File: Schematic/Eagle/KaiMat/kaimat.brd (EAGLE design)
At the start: 60.1 x 110.5 mm, 35 parts, among them IC1 MCP6004-E_P

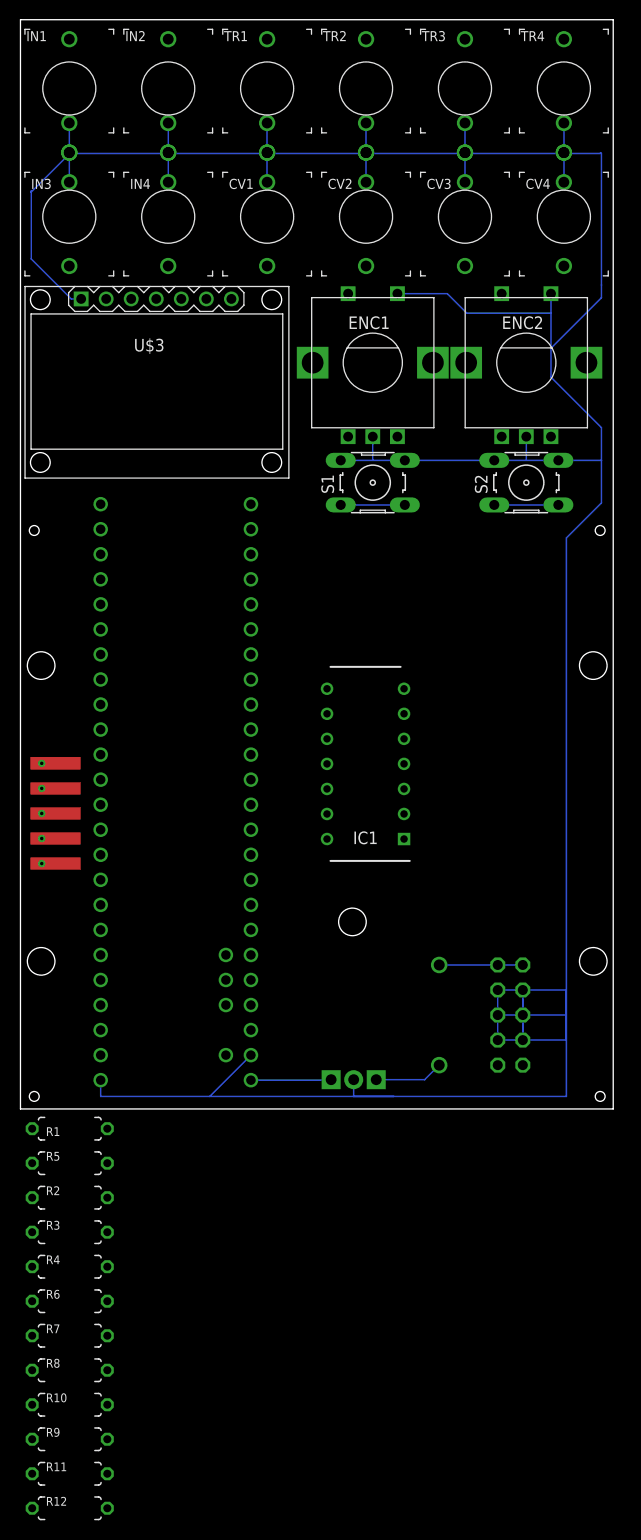
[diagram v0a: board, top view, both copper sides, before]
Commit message: improved schematic
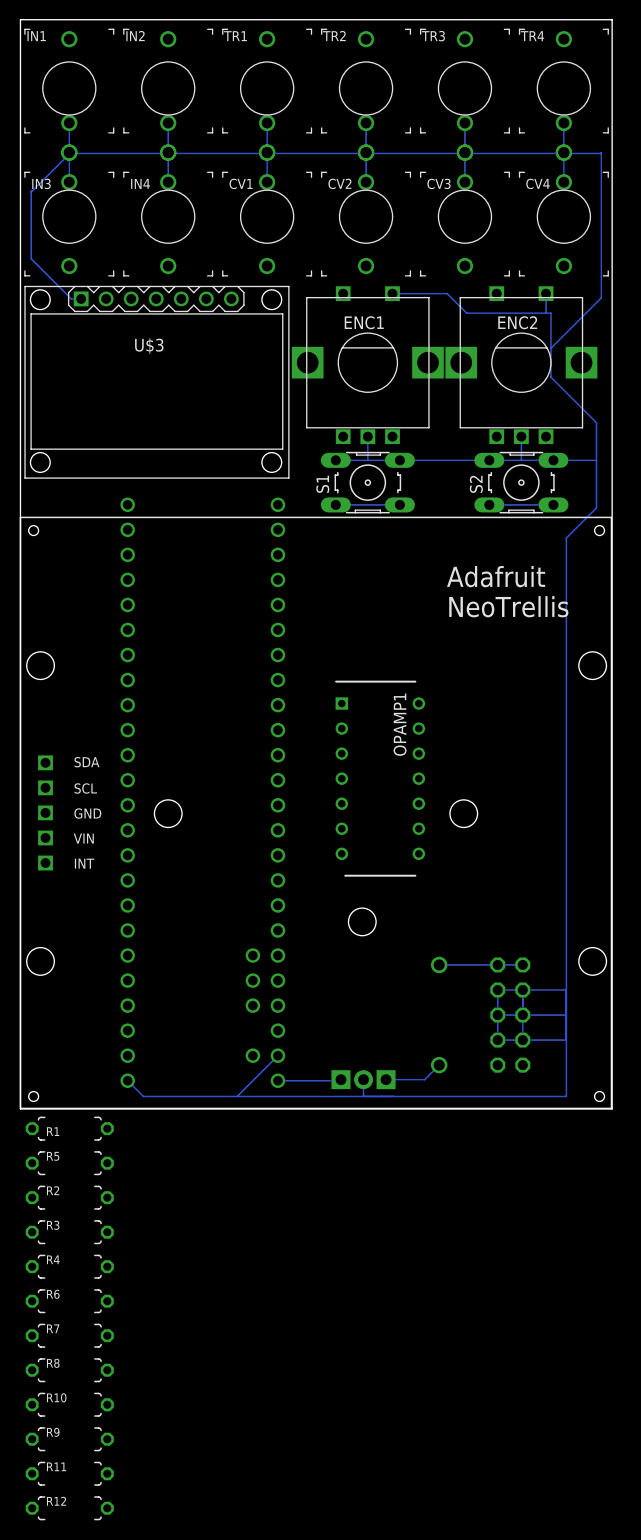
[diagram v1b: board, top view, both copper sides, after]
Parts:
- removed IC1: MCP6004-E_P, mcp6004-e_p:DIP781W56P254L1918H533Q14N
- removed JP1: (no value), microbuilder:5P_EDGECONNECT
- added OPAMP1: MCP6004-E_P, mcp6004-e_p:DIP781W56P254L1918H533Q14N
- added U$4: NEOTRELLISKAIMAT2, Adafruit Trellis:NEOTRELLISKAIMAT2
- moved U$1 2.74 mm to (18.5, 30.8)
- moved U$2 1.00 mm to (34.9, 12.6)
- moved ENC1 0.50 mm to (35.2, 75.7)
- moved ENC2 0.50 mm to (50.8, 75.7)
- moved S1 0.50 mm to (35.2, 63.5)
- moved S2 0.50 mm to (50.8, 63.5)
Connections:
- net +3V3: now also U$4.VIN
- net +5V: now also OPAMP1.4; no longer IC1.4
- net GND: now also OPAMP1.11, U$4.GND; no longer IC1.11
- net N$11: now also OPAMP1.5; no longer IC1.5
- net N$12: now also OPAMP1.13, OPAMP1.14; no longer IC1.13, IC1.14
- net N$13: now also OPAMP1.8, OPAMP1.9; no longer IC1.8, IC1.9
- net N$14: now also OPAMP1.3; no longer IC1.3
- net N$15: now also OPAMP1.10; no longer IC1.10
- net N$16: now also OPAMP1.12; no longer IC1.12
- net N$18: now also OPAMP1.1, OPAMP1.2; no longer IC1.1, IC1.2
- net N$4: now also OPAMP1.6, OPAMP1.7; no longer IC1.6, IC1.7
- net TRLSCL: now also U$4.SCL
- net TRLSDA: now also U$4.SDA
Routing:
- net GND: track 365.5 -> 358.2 mm
- net +5V: track 8.19 -> 6.51 mm
- net N$2: track 7.00 -> 6.00 mm
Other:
- board size 60.1 x 110.5 mm -> 60 x 110.5 mm
